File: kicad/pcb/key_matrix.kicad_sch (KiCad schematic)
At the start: 48 parts, among them SW1 EC_SW

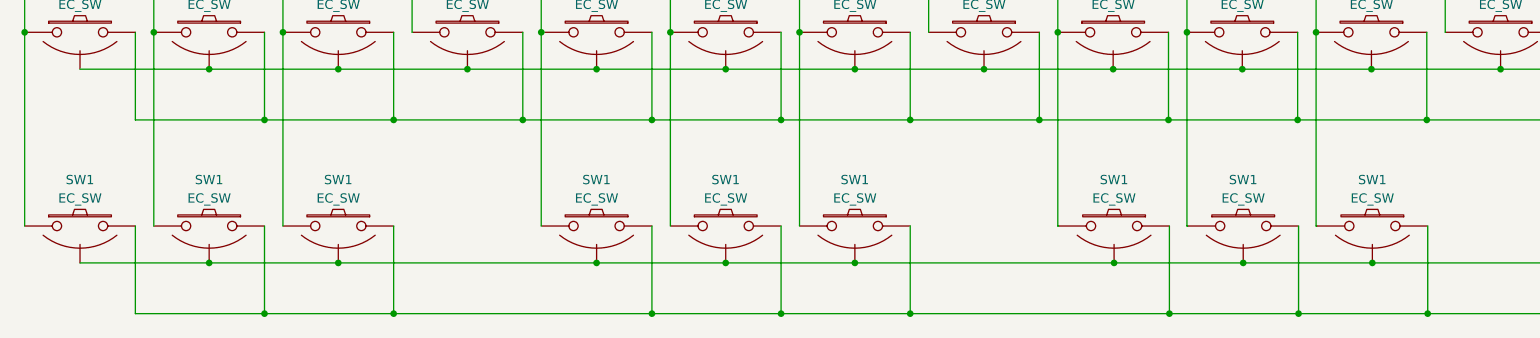
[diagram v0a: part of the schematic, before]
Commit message: update 3d model
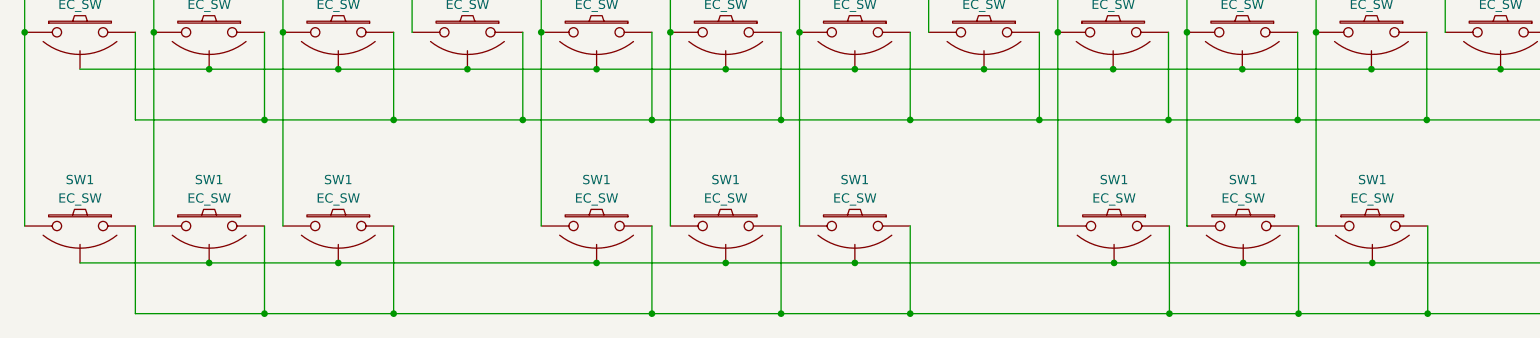
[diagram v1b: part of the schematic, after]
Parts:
- SW1: footprint capacitive_sensors:ecs_pad_1.75u_1.25u_combo -> capacitive_sensors:ecs_pad_combo_0.25u_offset
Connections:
- net COL0: now also SW1.2; no longer SW1.1
- net COL1: now also SW1.1; no longer SW1.2
- net COL10: now also SW1.1; no longer SW1.2
- net COL9: now also SW1.2; no longer SW1.1
- net ROW3: now also SW1.1, SW1.1, SW1.2, SW1.2; no longer SW1.1, SW1.1, SW1.2, SW1.2
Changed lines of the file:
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@@
     )
   )
-  (symbol (lib_id "cipulot_parts:EC_SW") (at 30.48 126.365 0) (unit 1)
+  (symbol (lib_id "cipulot_parts:EC_SW") (at 30.48 126.365 0) (mirror y) (unit 1)
     (in_bom no) (on_board yes) (dnp no)
     (property "Reference" "SW1" (at 30.48 120.015 0)
@@
     )
   )
-  (symbol (lib_id "cipulot_parts:EC_SW") (at 190.627 126.365 0) (unit 1)
+  (symbol (lib_id "cipulot_parts:EC_SW") (at 190.627 126.365 0) (mirror y) (unit 1)
     (in_bom no) (on_board yes) (dnp no)
     (property "Reference" "SW1" (at 190.627 120.015 0)
@@
       (effects (font (size 1.27 1.27)))
     )
-    (property "Footprint" "capacitive_sensors:ecs_pad_1.75u_1.25u_combo" (at 30.48 73.025 0)
+    (property "Footprint" "capacitive_sensors:ecs_pad_combo_0.25u_offset" (at 30.48 73.025 0)
       (effects (font (size 1.27 1.27)) hide)
     )
@@
     )
   )
-  (symbol (lib_id "cipulot_parts:EC_SW") (at 48.26 126.365 0) (mirror y) (unit 1)
+  (symbol (lib_id "cipulot_parts:EC_SW") (at 48.26 126.365 0) (unit 1)
     (in_bom no) (on_board yes) (dnp no)
     (property "Reference" "SW1" (at 48.26 120.015 0)
@@
     )
   )
-  (symbol (lib_id "cipulot_parts:EC_SW") (at 208.407 126.365 0) (mirror y) (unit 1)
+  (symbol (lib_id "cipulot_parts:EC_SW") (at 208.407 126.365 0) (unit 1)
     (in_bom no) (on_board yes) (dnp no)
     (property "Reference" "SW1" (at 208.407 120.015 0)
